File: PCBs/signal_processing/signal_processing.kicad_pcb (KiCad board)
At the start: 2 copper layers, 75 x 36 mm, 135 parts, among them IC1 AD8066, IC2 AD8066, IC3 AD8066, IC4 AD8066, IC5 ADG701, IC6 LT1713, IC7 LT1713, J1 CON-SMA-EDGE-S, J2 874380443, J3 874380443, J4 874380443, J5 CON-SMA-EDGE-S, J6 CON-SMA-EDGE-S

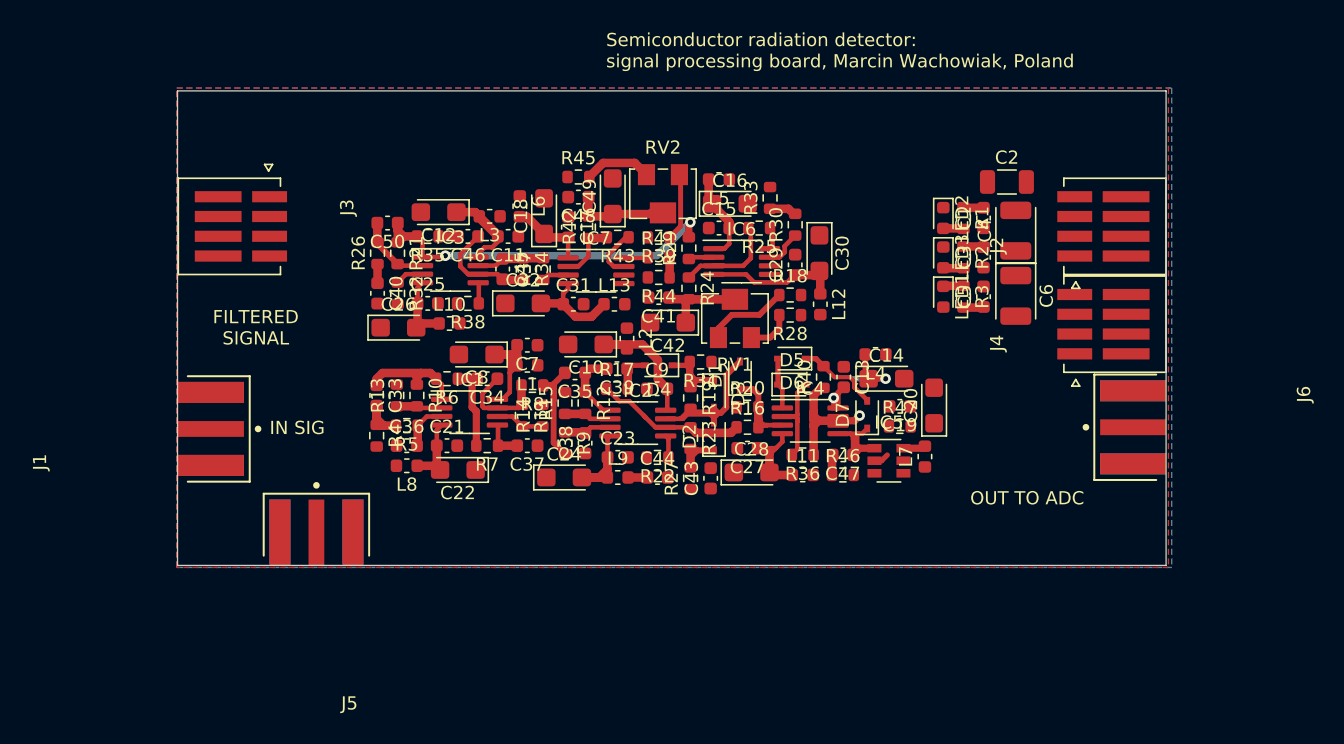
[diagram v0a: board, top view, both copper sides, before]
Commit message: finished pcbs
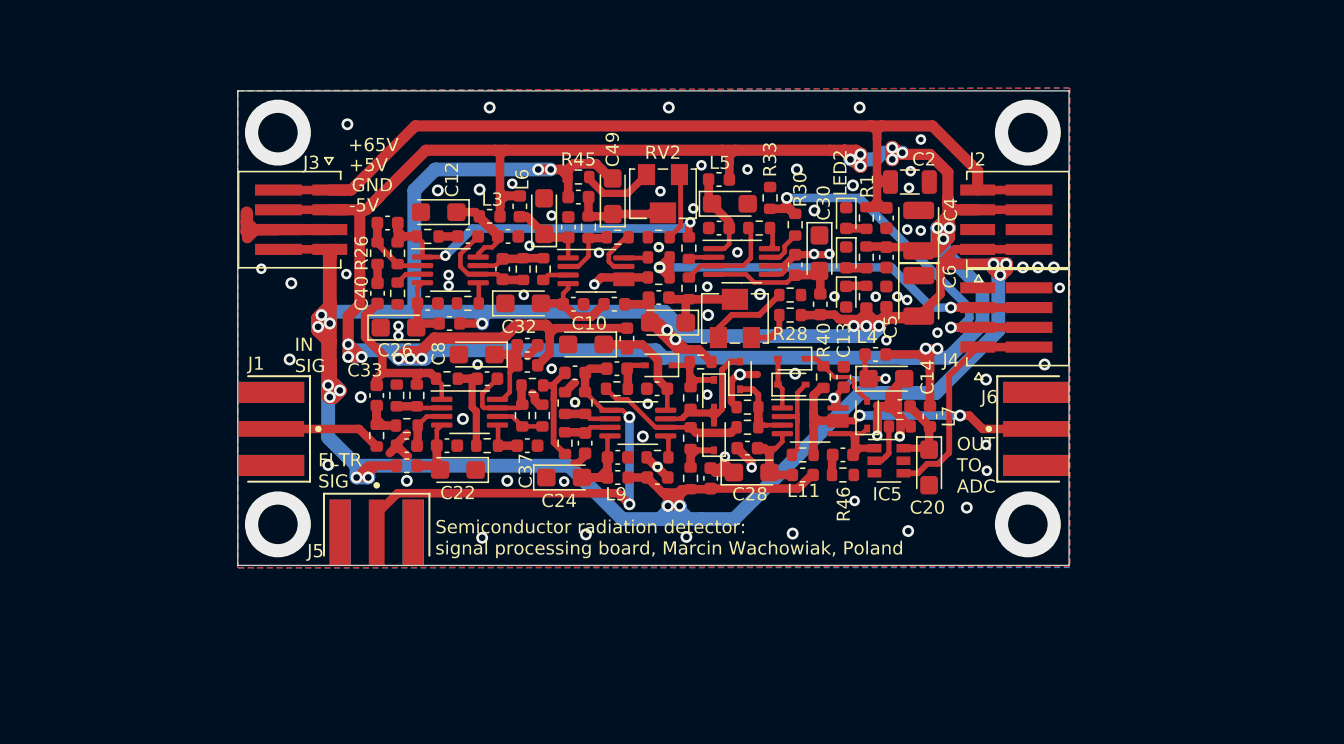
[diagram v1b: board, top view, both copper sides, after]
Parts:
- moved J4 7.38 mm to (174.8, 104.2)
- moved J2 7.38 mm to (174.8, 96.8)
- moved J6 7.37 mm to (183.4, 112.6)
- moved C1 7.37 mm to (164.8, 96.6)
- moved C2 7.37 mm to (166.6, 93.9)
- moved C3 7.37 mm to (164.8, 99.6)
- moved C4 7.37 mm to (167.2, 97.6)
- moved C5 7.37 mm to (164.8, 102.6)
- moved C6 7.37 mm to (167.2, 102.6)
- moved LED1 7.37 mm to (161.7, 102.6)
- moved LED2 7.37 mm to (161.7, 96.6)
- moved LED3 7.37 mm to (161.7, 99.6)
- moved R1 7.37 mm to (163.3, 96.6)
- moved R2 7.37 mm to (163.3, 99.6)
- moved R3 7.37 mm to (163.3, 102.6)
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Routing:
- net -5V: track 3.00 -> 297.3 mm, vias 0 -> 21
- net +5V: track 1.54 -> 250.0 mm, vias 0 -> 17
- net /+65V: track 1.54 -> 76.6 mm
- net GND: track 0.00 -> 63.8 mm, vias 0 -> 83
- net /RISING_SLOPE: track 1.52 -> 33.8 mm, vias 0 -> 2
- net /FILTERED_SIGNAL: track 5.29 -> 35.2 mm, vias 0 -> 2
- net /PULSE_DURATION: track 1.94 -> 31.0 mm, vias 0 -> 2
- net /RESET: track 0.00 -> 16.9 mm
- net /ADC: track 11.2 -> 25.0 mm, vias 1 -> 2
- net /SIGNAL_INPUT: track 0.00 -> 8.55 mm
- net /FAST_FILTERED_SIG: track 8.11 -> 14.3 mm
- net Net-(C19-Pad2): track 1.69 -> 5.63 mm
- net Net-(IC5-Pad2): track 1.15 -> 3.59 mm
- net Net-(C13-Pad2): track 9.93 -> 12.0 mm
- net Net-(D1-Pad2): track 14.3 -> 15.5 mm
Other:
- board size 75 x 36 mm -> 63.1 x 36 mm
- board text added: "FLTR SIG"
- board text removed: "FILTERED SIGNAL"
